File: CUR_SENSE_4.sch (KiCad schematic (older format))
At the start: 7 parts

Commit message: blubb
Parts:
- removed D5, D6, D7, D9: 3V, Diodes_SMD:SOD-323, symbol D_Schottky_Small
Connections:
- wire segments 32 -> 22
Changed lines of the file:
@@
 Connection ~ 1500 1600
 $Comp
-L GND #PWR037
+L GND #PWR038
 U 1 1 57A226A1
 P 1550 1650
-F 0 "#PWR037" H 1550 1400 50  0001 C CNN
+F 0 "#PWR038" H 1550 1400 50  0001 C CNN
 F 1 "GND" H 1550 1500 50  0000 C CNN
 F 2 "" H 1550 1650 50  0000 C CNN
@@
 Connection ~ 1550 1600
 Wire Wire Line
-	2250 1200 2250 1050
-Wire Wire Line
 	2150 1050 2800 1050
-Wire Wire Line
-	2350 950  2350 1200
 Wire Wire Line
 	2150 950  2800 950
 Wire Wire Line
-	2450 850  2450 1200
-Wire Wire Line
 	2150 850  2800 850
-Wire Wire Line
-	2550 750  2550 1200
 Wire Wire Line
 	2150 750  2800 750
@@
 Text HLabel 2800 1050 2    60   Output ~ 0
 OUT_4
-Connection ~ 2250 1050
-Connection ~ 2350 950
-Connection ~ 2450 850
-Connection ~ 2550 750
-Wire Wire Line
-	2550 1500 2550 1400
-Wire Wire Line
-	2250 1500 2550 1500
-Wire Wire Line
-	2250 1500 2250 1400
-Wire Wire Line
-	2350 1400 2350 1500
-Connection ~ 2350 1500
-Wire Wire Line
-	2450 1400 2450 1500
-Connection ~ 2450 1500
-$Comp
-L GND #PWR038
-U 1 1 57A22B7D
-P 2400 1600
-F 0 "#PWR038" H 2400 1350 50  0001 C CNN
-F 1 "GND" H 2400 1450 50  0000 C CNN
-F 2 "" H 2400 1600 50  0000 C CNN
-F 3 "" H 2400 1600 50  0000 C CNN
-	1    2400 1600
-	1    0    0    -1
-$EndComp
-$Comp
-L D_Schottky_Small D5
-U 1 1 57A22C08
-P 2250 1300
-F 0 "D5" H 2200 1380 50  0000 L CNN
-F 1 "3V" H 2100 1250 50  0000 L CNN
-F 2 "Diodes_SMD:SOD-323" V 2250 1300 50  0001 C CNN
-F 3 "" V 2250 1300 50  0000 C CNN
-	1    2250 1300
-	0    1    1    0
-$EndComp
-$Comp
-L D_Schottky_Small D6
-U 1 1 57A22CDB
-P 2350 1300
-F 0 "D6" H 2300 1380 50  0000 L CNN
-F 1 "3V" H 2200 1250 50  0000 L CNN
-F 2 "Diodes_SMD:SOD-323" V 2350 1300 50  0001 C CNN
-F 3 "" V 2350 1300 50  0000 C CNN
-	1    2350 1300
-	0    1    1    0
-$EndComp
-$Comp
-L D_Schottky_Small D7
-U 1 1 57A22D00
-P 2450 1300
-F 0 "D7" H 2400 1380 50  0000 L CNN
-F 1 "3V" H 2300 1250 50  0000 L CNN
-F 2 "Diodes_SMD:SOD-323" V 2450 1300 50  0001 C CNN
-F 3 "" V 2450 1300 50  0000 C CNN
-	1    2450 1300
-	0    1    1    0
-$EndComp
-$Comp
-L D_Schottky_Small D9
-U 1 1 57A22D28
-P 2550 1300
-F 0 "D9" H 2500 1380 50  0000 L CNN
-F 1 "3V" H 2400 1250 50  0000 L CNN
-F 2 "Diodes_SMD:SOD-323" V 2550 1300 50  0001 C CNN
-F 3 "" V 2550 1300 50  0000 C CNN
-	1    2550 1300
-	0    1    1    0
-$EndComp
-Wire Wire Line
-	2400 1600 2400 1500
-Connection ~ 2400 1500
 $EndSCHEMATC

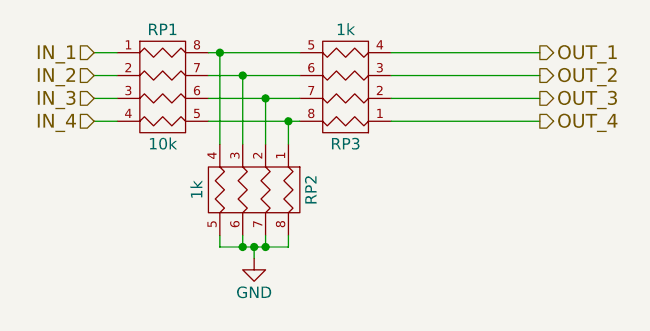
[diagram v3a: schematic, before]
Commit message: updated stuff
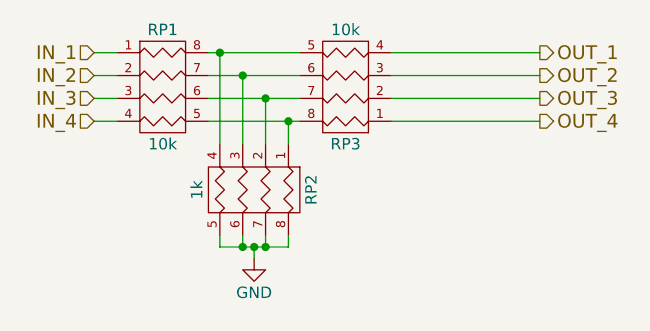
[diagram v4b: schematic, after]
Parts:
- RP3: value 1k -> 10k
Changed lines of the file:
@@
 $Descr A4 11693 8268
 encoding utf-8
-Sheet 7 13
+Sheet 6 12
 Title ""
 Date ""
@@
 P 1950 700
 F 0 "RP3" H 1950 1150 50  0000 C CNN
-F 1 "1k" H 1950 650 50  0000 C CNN
+F 1 "10k" H 1950 650 50  0000 C CNN
 F 2 "Resistors_SMD:R_Array_Concave_4x0603" H 1950 700 50  0001 C CNN
 F 3 "" H 1950 700 50  0000 C CNN
